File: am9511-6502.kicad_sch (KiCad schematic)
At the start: 13 parts, among them U1 AM9511A, U2 ATF16V8B, U3 74HC112, U4 ADA-TPS61040, U5 74HC123, X1 4 MHz

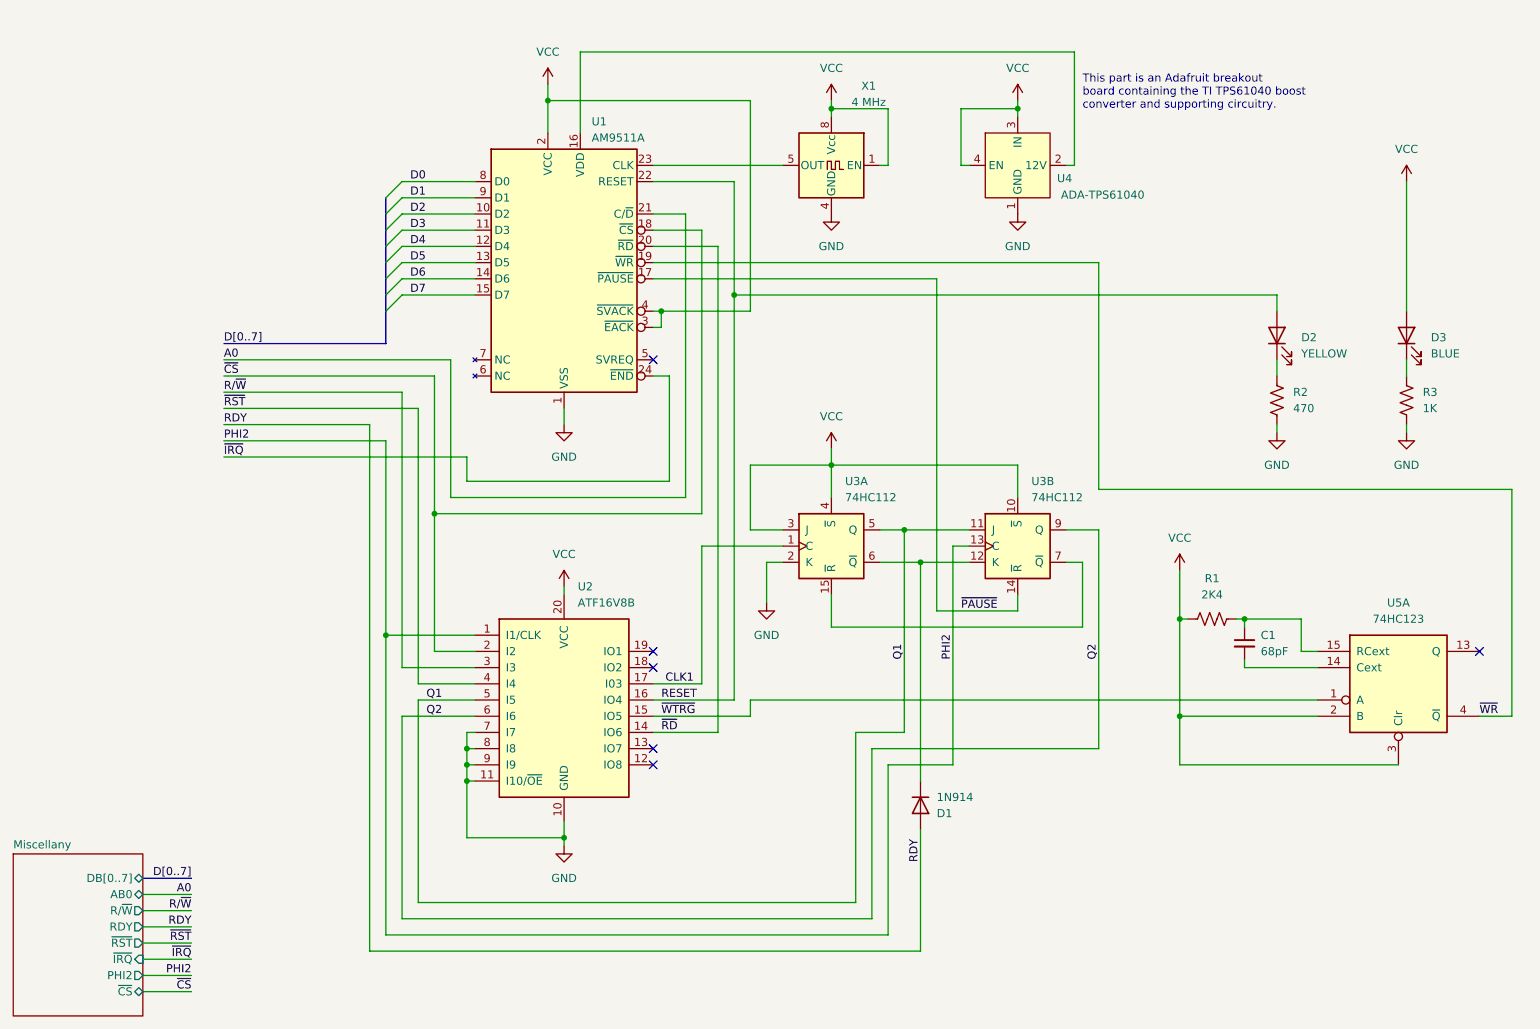
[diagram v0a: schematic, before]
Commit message: Initial PAL-2 version
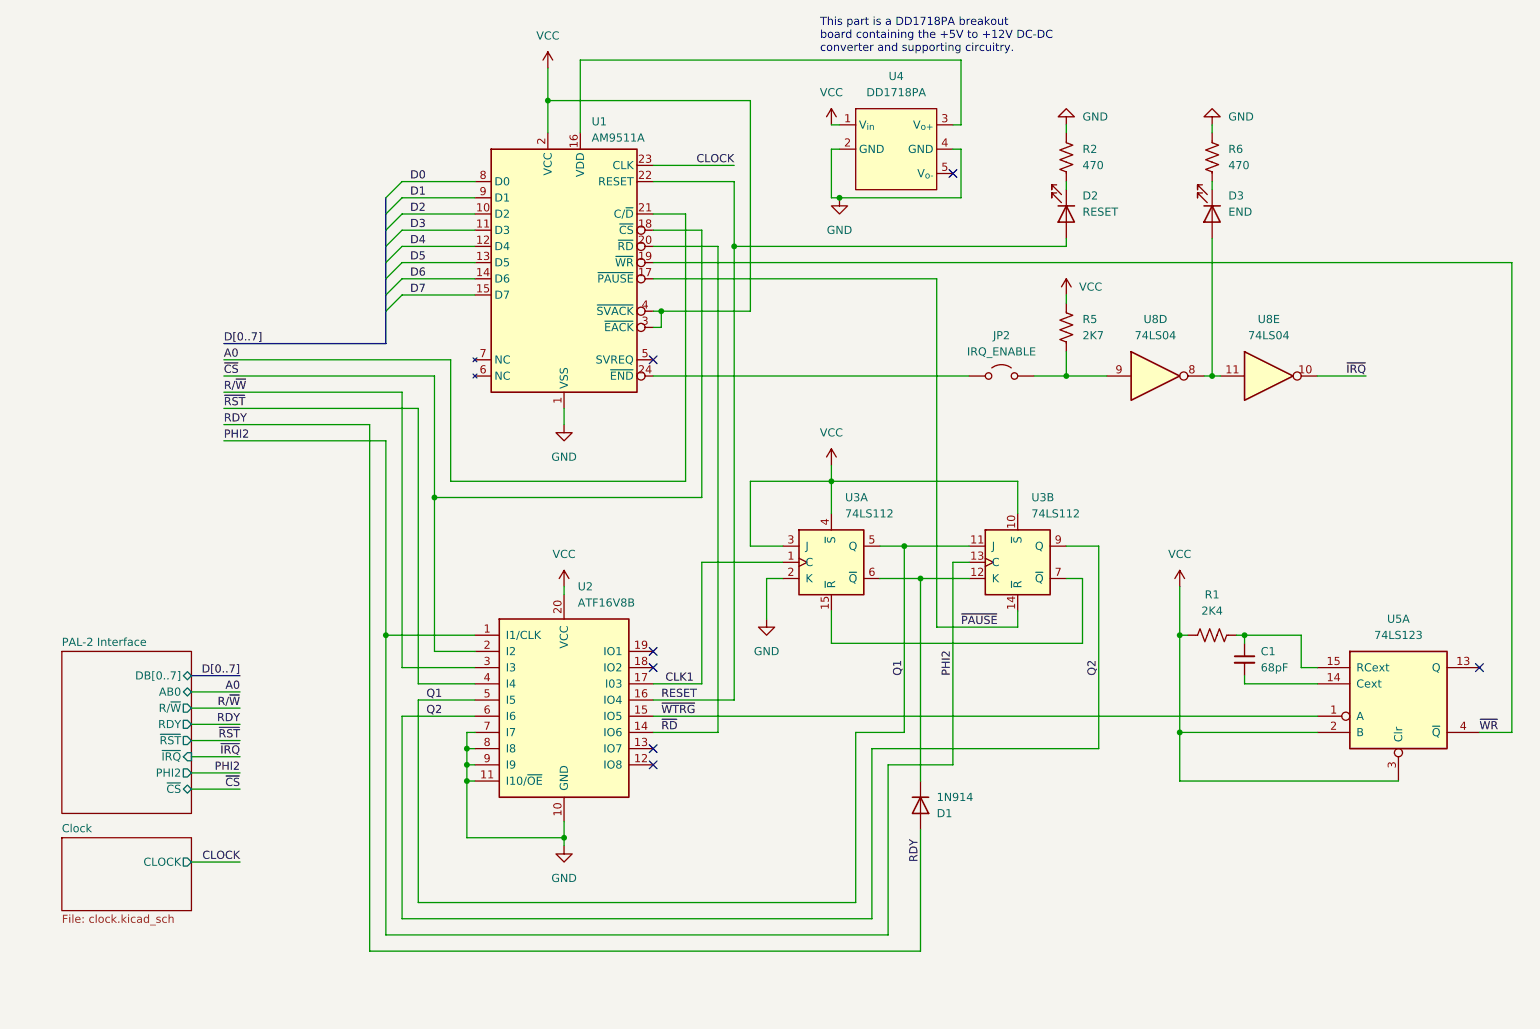
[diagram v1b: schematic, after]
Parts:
- removed R3: 1K, Resistor_THT:R_Axial_DIN0207_L6.3mm_D2.5mm_P7.62mm_Horizontal, symbol Device:R_US
- removed U4: ADA-TPS61040, am9511-6502-footprints:ADA-TPS61040, symbol am9511-6502-symbols:ADA-TPS61040
- removed X1: 4 MHz, Oscillator:Oscillator_DIP-8, symbol Oscillator:CXO_DIP8
- added JP2: IRQ_ENABLE, Connector_PinHeader_2.54mm:PinHeader_1x02_P2.54mm_Vertical, symbol Jumper:Jumper_2_Open
- added R5: 2K7, Resistor_THT:R_Axial_DIN0207_L6.3mm_D2.5mm_P7.62mm_Horizontal, symbol Device:R_US
- added R6: 470, Resistor_THT:R_Axial_DIN0207_L6.3mm_D2.5mm_P7.62mm_Horizontal, symbol Device:R_US
- added U4: DD1718PA, am9511-6502-footprints:DD1718PA, symbol am9511-6502-symbols:DD1718PA
- added U8: 74LS04, Package_DIP:DIP-14_W7.62mm_Socket, symbol 74xx:74HC04
- D2: value YELLOW -> RESET
- D3: value BLUE -> END
- U3: value 74HC112 -> 74LS112
- U5: value 74HC123 -> 74LS123
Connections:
- net GND: now also R2.1, R6.1, U4.2 (GND), U4.4 (GND); no longer R2.2
- net VCC: now also R5.1, U4.1 (V_{in}); no longer D3.2 (A)
- net ~{IRQ}: now also U8.10; no longer U1.24 (~{END})
- net at D2.1 (K): now also R2.2; no longer R2.1
- net at U1.16 (VDD): now also U4.3 (V_{o+})
- net at D3.1 (K): now also R6.2
- net CLOCK: now reaches U1.23 (CLK)
- new net: D3.2 (A), U8.11, U8.8
- new net: JP2.2 (B), R5.2, U8.9
- new net: JP2.1 (A), U1.24 (~{END})
- no-connect marks 6 -> 7
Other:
- sheet Miscellany renamed PAL-2 Interface
- added sheet Clock (clock.kicad_sch)
- note added: "This part is a DD1718PA breakout board containing the +5V to +12V DC-DC converter and supporting circuitry."
- note removed: "This part is an Adafruit breakout board containing the TI TPS61040 boost converter and supporting circuitry."
- moved on the sheet: C1, D2, R1, R2, U3A, U3B, U5A

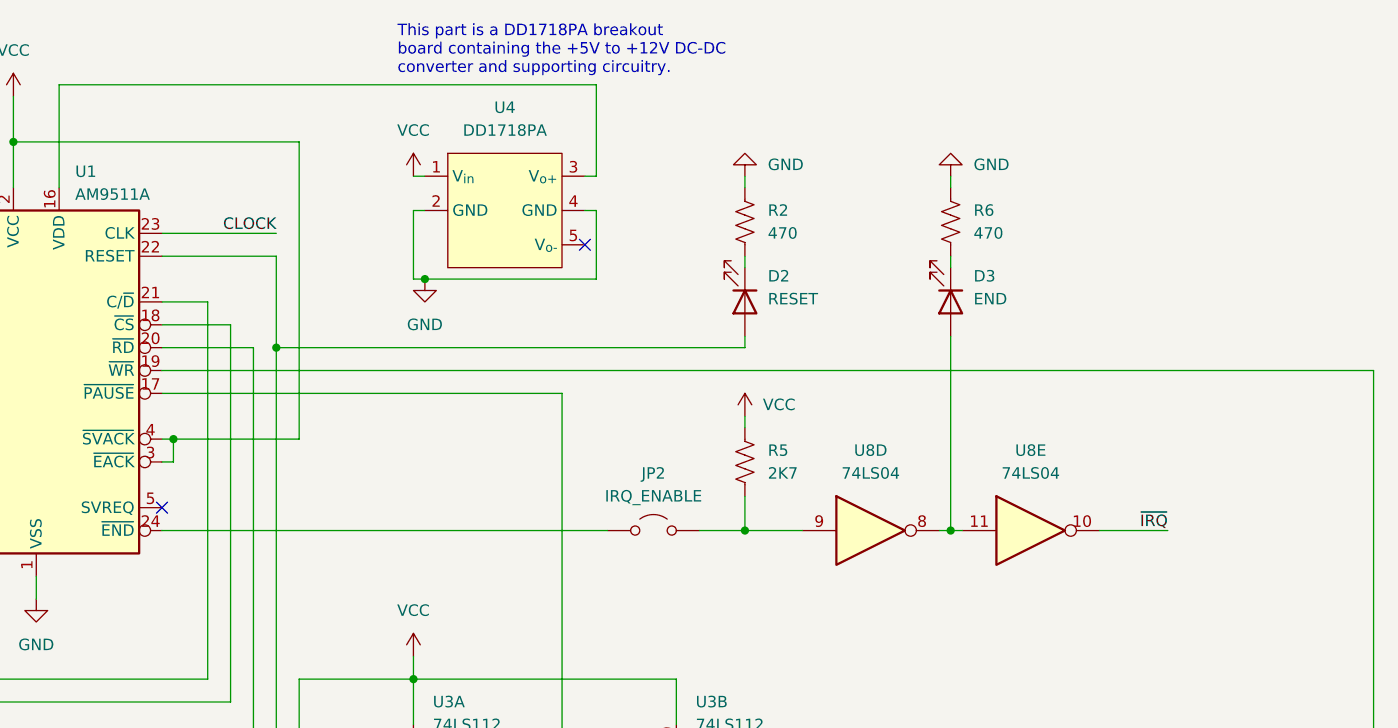
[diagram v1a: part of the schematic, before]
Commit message: First manufacturing prototype
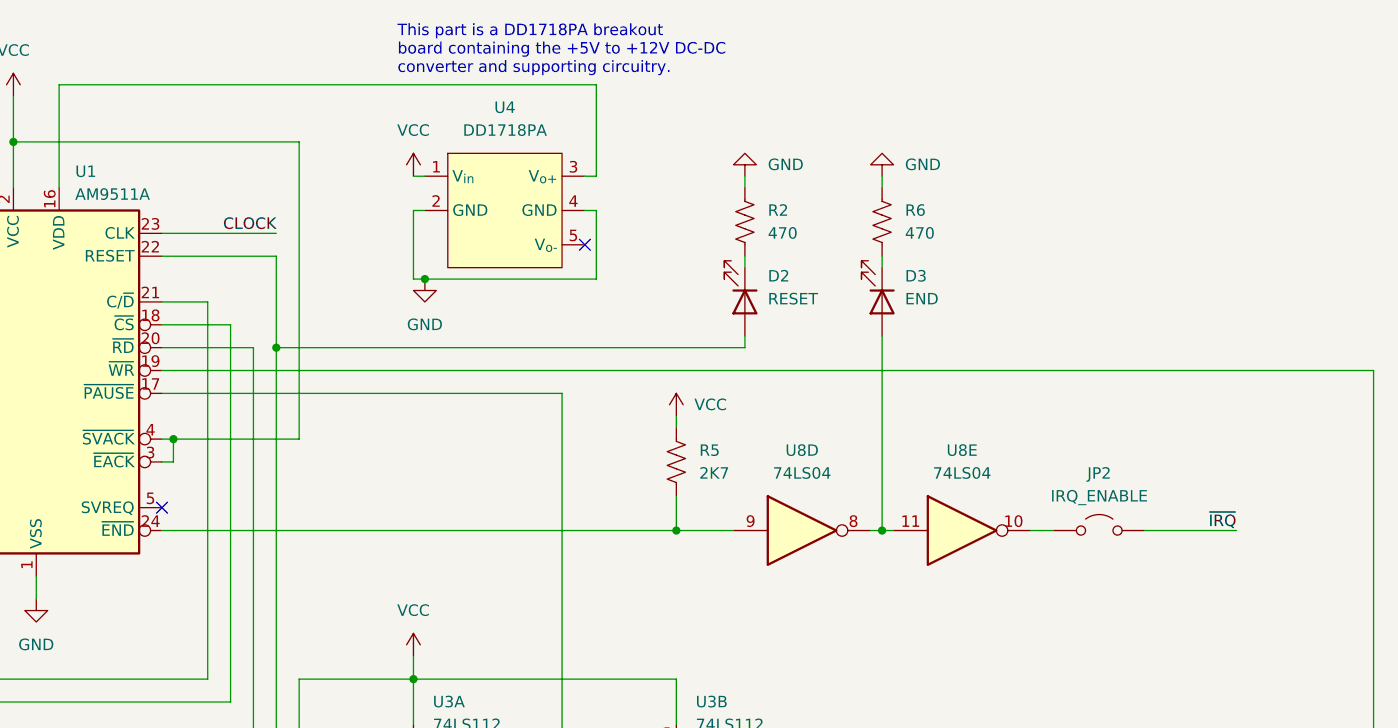
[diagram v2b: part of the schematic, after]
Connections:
- net ~{IRQ}: now also JP2.1 (A); no longer U8.10
- net at R5.2, U8.9: now also U1.24 (~{END}); no longer JP2.2 (B)
- new net: JP2.2 (B), U8.10
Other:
- moved on the sheet: D3, JP2, R5, R6, U8D, U8E
